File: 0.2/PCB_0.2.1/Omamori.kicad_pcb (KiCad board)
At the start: 2 copper layers, 25 x 35 mm, 34 parts, among them J1 Conn_01x04_Female, Q1 IRLML0030, U1 BQ25504, U2 TPS61222DCK, U3 ATtiny85, U4 TS-1233

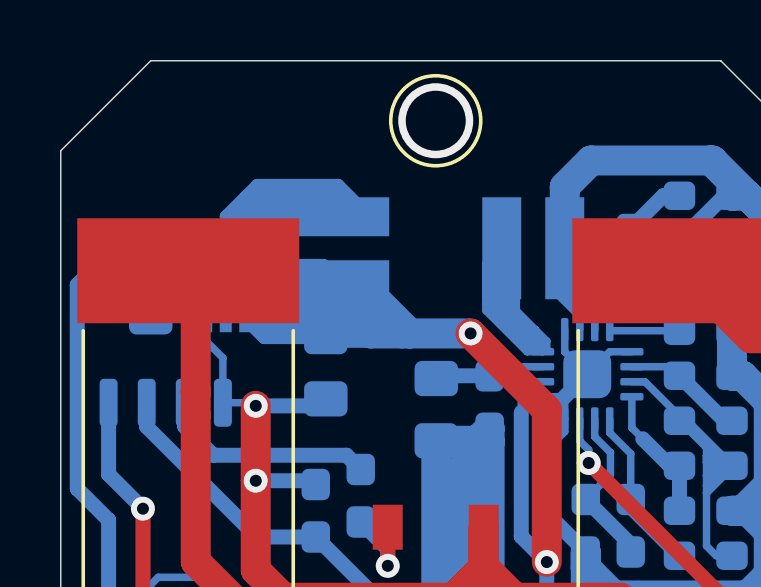
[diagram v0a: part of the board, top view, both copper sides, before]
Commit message: Added Interactive BOM. Updated Gerber Files.
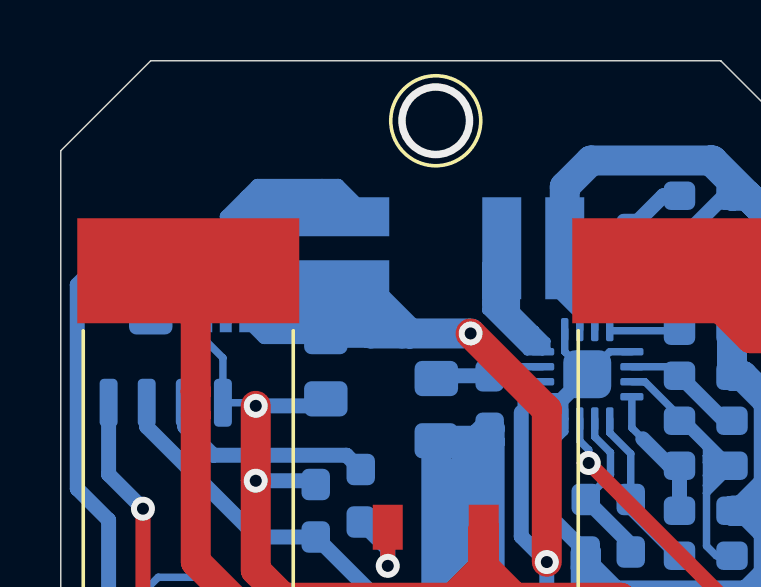
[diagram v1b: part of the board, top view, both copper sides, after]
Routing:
- net /Vbat: track 86.7 -> 84.7 mm
